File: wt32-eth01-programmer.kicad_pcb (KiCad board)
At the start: 2 copper layers, 31.8 x 76.2 mm, 23 parts, among them J1 USB_C_Receptacle_USB2.0, Q1 S8050, Q2 S8050, SW1 SW_DPST_x2, U1 AMS1117-3.3, U2 CH340G, U3 WT32-ETH0-Board, Y1 12Mhz

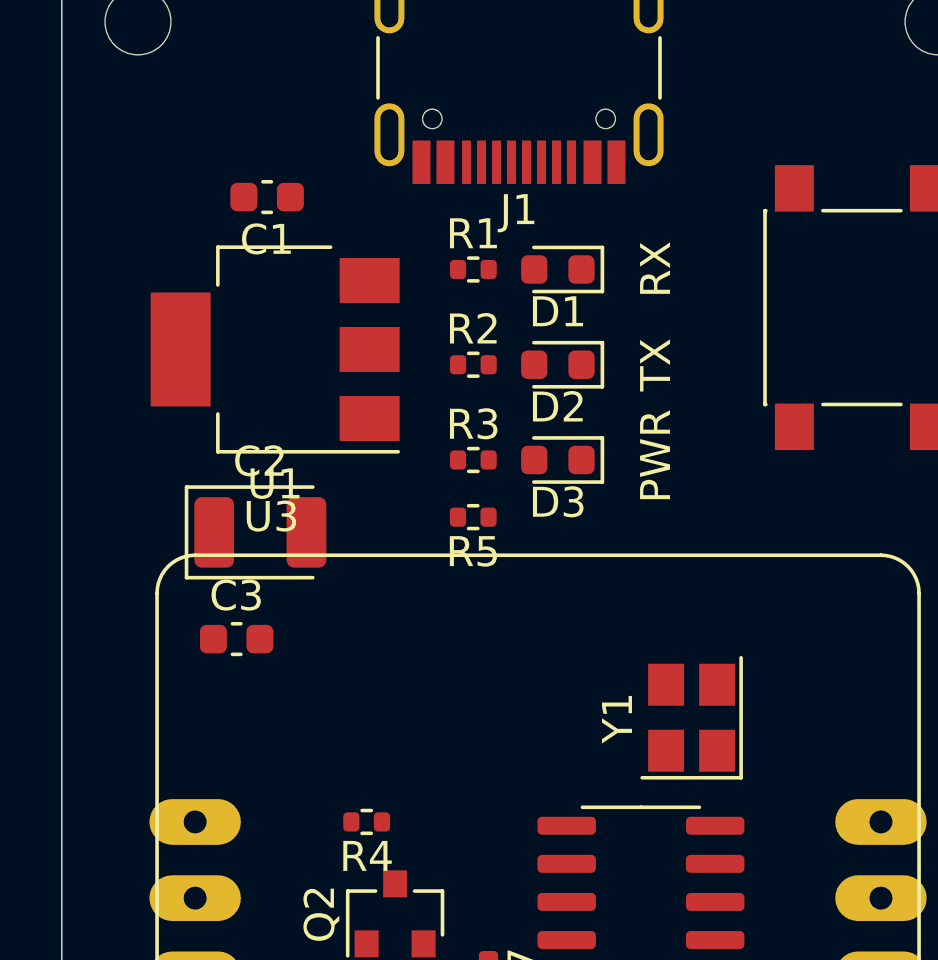
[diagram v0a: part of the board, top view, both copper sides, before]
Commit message: layout
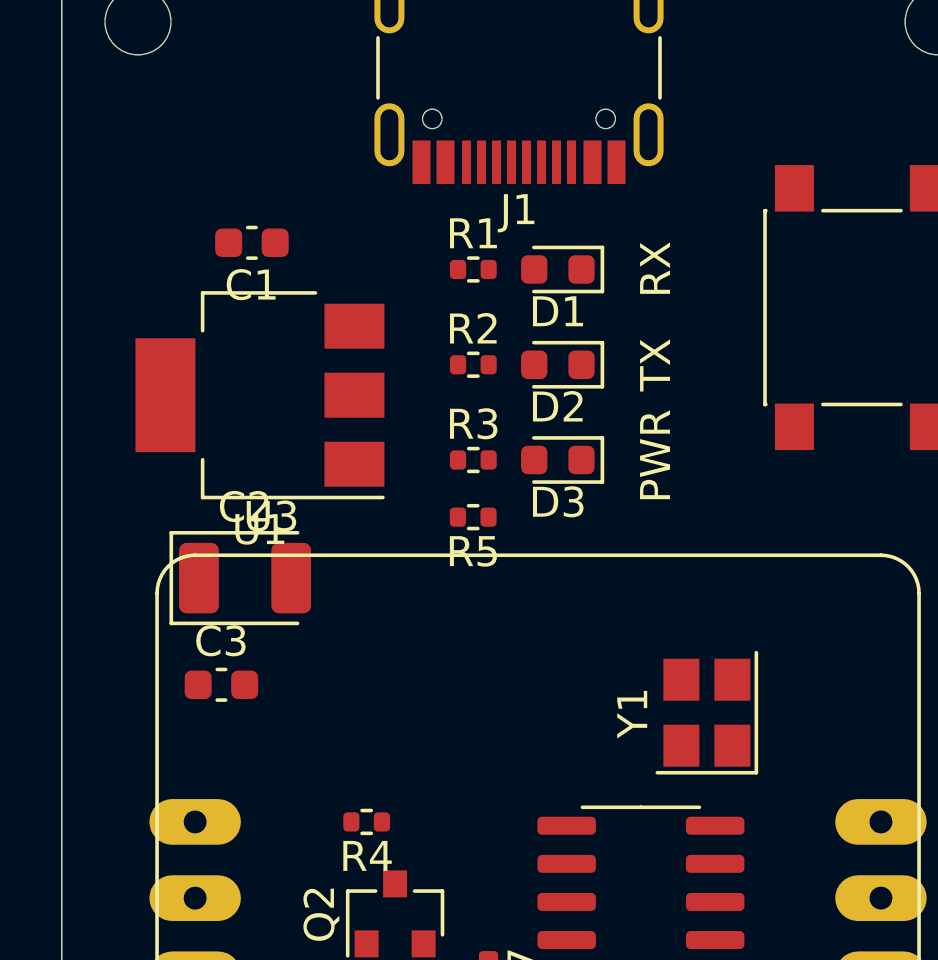
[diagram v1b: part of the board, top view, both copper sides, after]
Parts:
- moved C1 1.61 mm to (57.1, 54.4)
- moved C2 1.61 mm to (56.9, 65.5)
- moved C3 1.61 mm to (56.1, 69.1)
- moved U1 1.61 mm to (57.4, 59.4)
- moved Y1 0.54 mm to (72.3, 70.0)
